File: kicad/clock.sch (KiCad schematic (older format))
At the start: 26 parts, among them SW1 SW_Push, U1 74HC04, U10 Discrete_NAND, U11 7SEGMENT_CC, U12 4543, U13 7SEGMENT_CC, U14 4543, U15 Discrete_NAND, U16 Discrete_NAND, U17 7SEGMENT_CC, U2 74LS390, U3 CD4060, U4 4543, U5 7SEGMENT_CC, U6 4027, U7 74LS390, U8 74LS390, U9 4543, Y1 32768

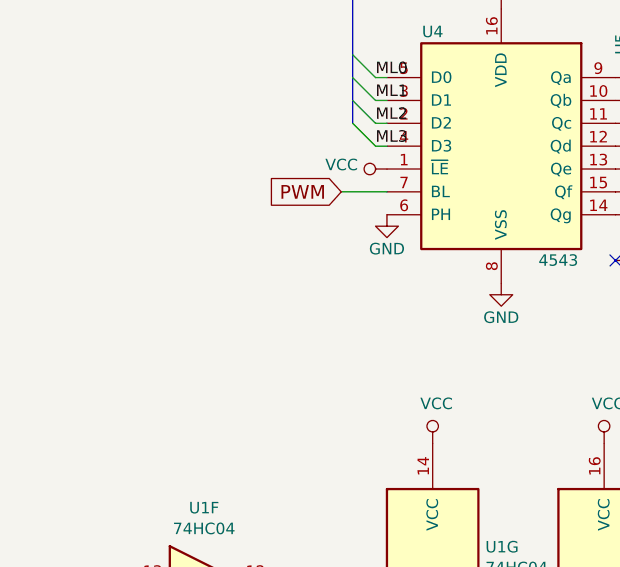
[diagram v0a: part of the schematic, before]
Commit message: Routing done: need board edges
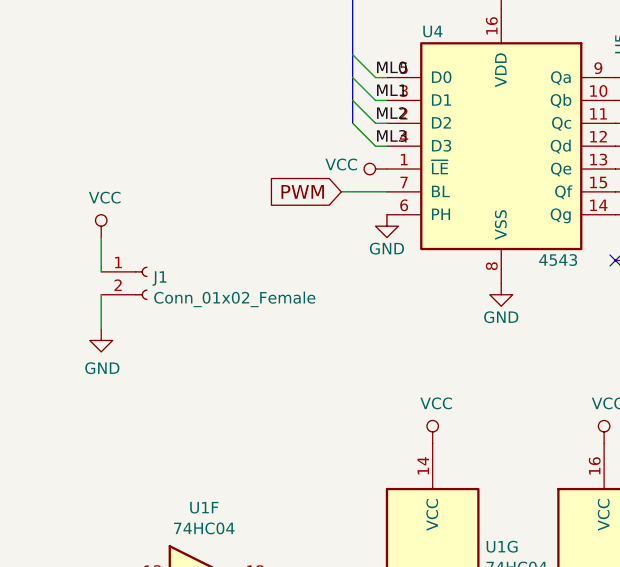
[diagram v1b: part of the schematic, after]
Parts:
- added J1: Conn_01x02_Female, Wire_Pads:SolderWirePad_2x_1mmDrill, symbol Connector:Conn_01x02_Female
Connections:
- net GND: now also J1.2 (Pin_2)
- net VCC: now also J1.1 (Pin_1)
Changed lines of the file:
@@
 Wire Wire Line
 	3150 900  3200 900
+$Comp
+L power:VCC #PWR088
+U 1 1 5D784885
+P 850 5550
+F 0 "#PWR088" H 850 5400 50  0001 C CNN
+F 1 "VCC" H 867 5723 50  0000 C CNN
+F 2 "" H 850 5550 50  0001 C CNN
+F 3 "" H 850 5550 50  0001 C CNN
+	1    850  5550
+	1    0    0    -1
+$EndComp
+$Comp
+L power:GND #PWR089
+U 1 1 5D7851FE
+P 850 5950
+F 0 "#PWR089" H 850 5700 50  0001 C CNN
+F 1 "GND" H 855 5777 50  0000 C CNN
+F 2 "" H 850 5950 50  0001 C CNN
+F 3 "" H 850 5950 50  0001 C CNN
+	1    850  5950
+	1    0    0    -1
+$EndComp
+$Comp
+L Connector:Conn_01x02_Female J1
+U 1 1 5D777D7F
+P 1050 5700
+F 0 "J1" H 1078 5676 50  0000 L CNN
+F 1 "Conn_01x02_Female" H 1078 5585 50  0000 L CNN
+F 2 "Wire_Pads:SolderWirePad_2x_1mmDrill" H 1050 5700 50  0001 C CNN
+F 3 "~" H 1050 5700 50  0001 C CNN
+	1    1050 5700
+	1    0    0    -1
+$EndComp
+Wire Wire Line
+	850  5950 850  5800
+Wire Wire Line
+	850  5700 850  5550
 Wire Bus Line
 	8950 4100 8950 5050
